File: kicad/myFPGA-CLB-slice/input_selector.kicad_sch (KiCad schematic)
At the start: 26 parts, among them U1 74AHCT595, U32 74LS153, U33 74LS153, U34 74LS153, U35 74LS153

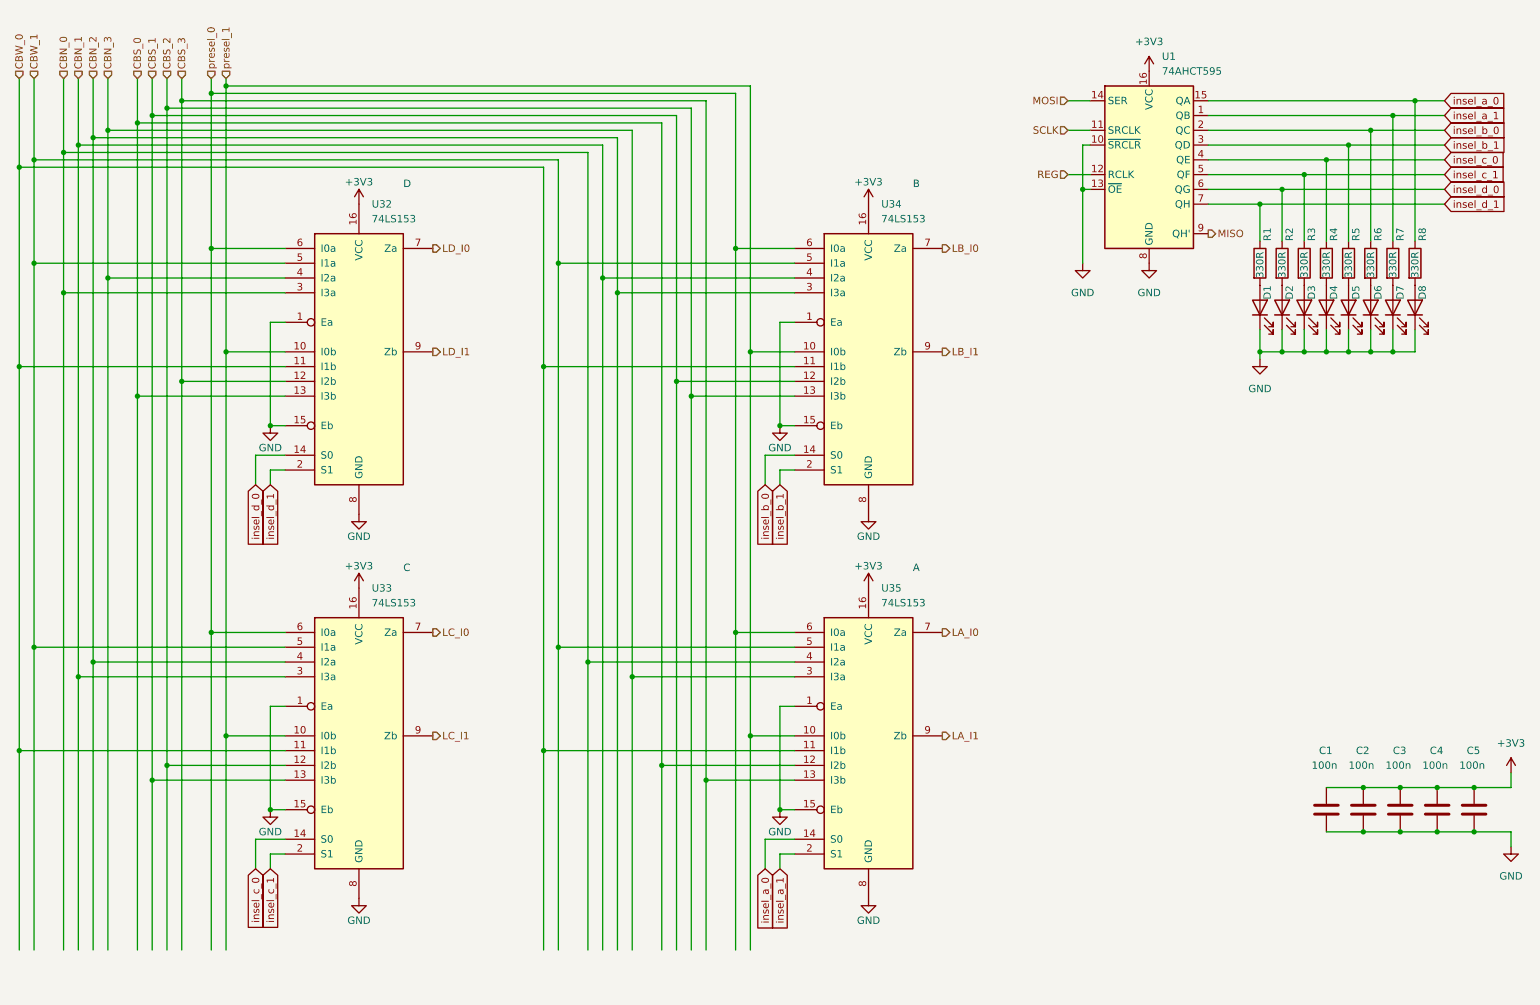
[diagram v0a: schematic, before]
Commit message: fixed kicad names, updated architecure, started CBv
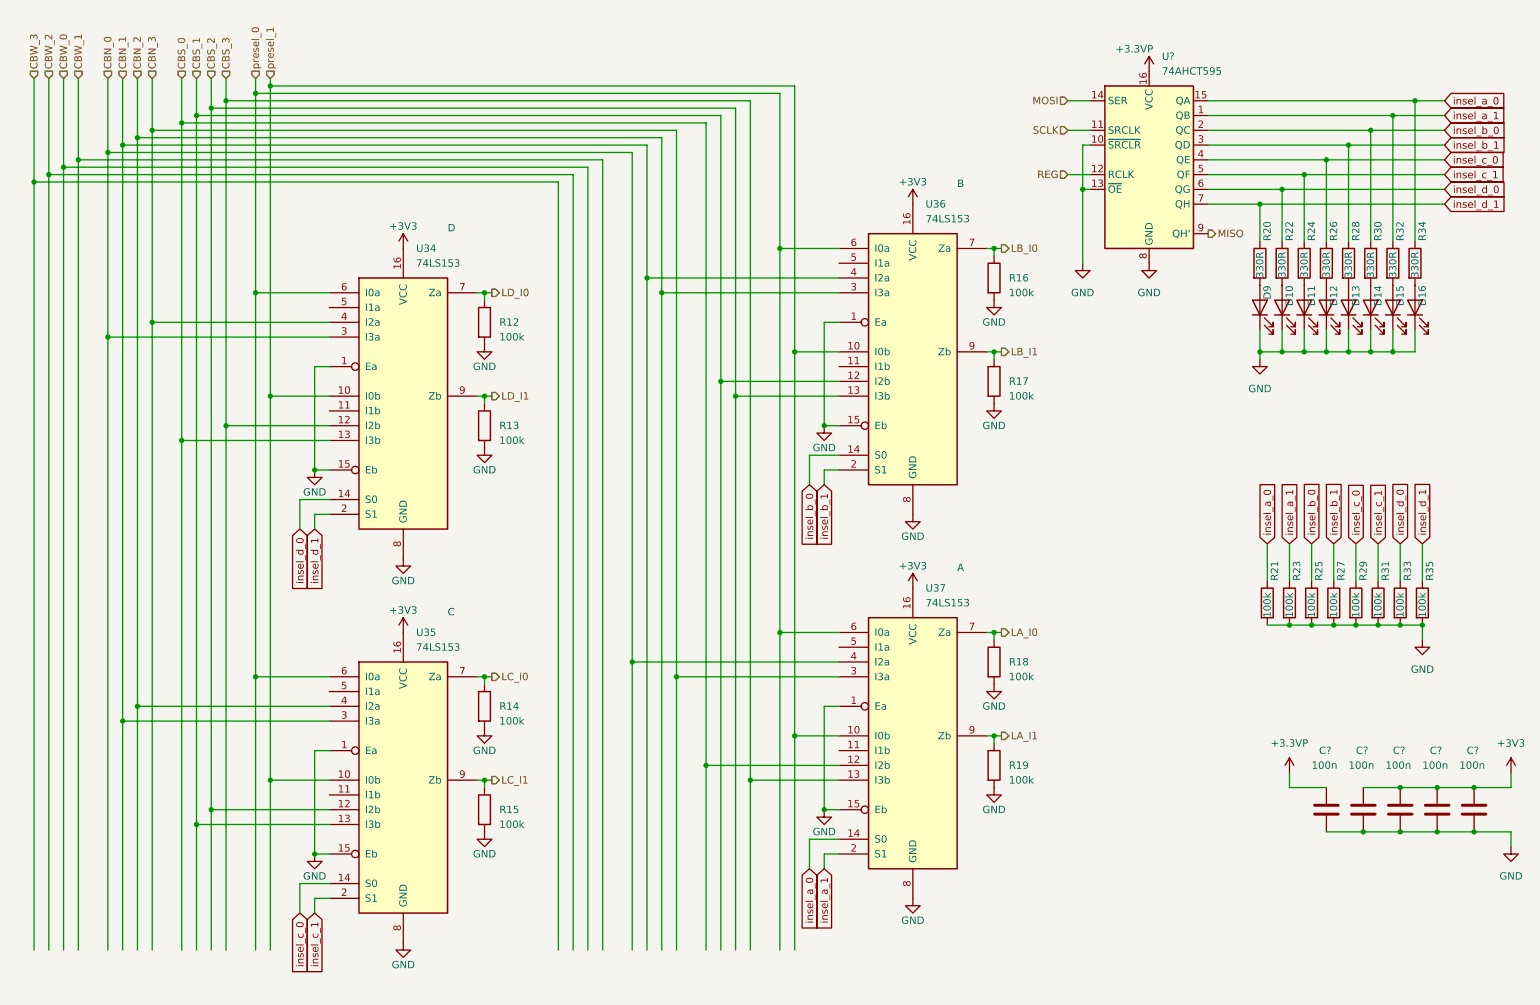
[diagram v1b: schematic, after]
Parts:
- added R12, R13, R14, R15, R16, R17, R18, R19, R21, R23, R25, R27, R29, R31, R33, R35: 100k, Resistor_SMD:R_0805_2012Metric, symbol Device:R
- C?: renamed from C4; Dielectric (none) -> X7R; JLCPCB Part # (none) -> C49678; Part Nr. (none) -> CC0805KRX7R9BB104; Voltage (none) -> 50V
- C?: renamed from C3; Dielectric (none) -> X7R; JLCPCB Part # (none) -> C49678; Part Nr. (none) -> CC0805KRX7R9BB104; Voltage (none) -> 50V
- C?: renamed from C1; Dielectric (none) -> X7R; JLCPCB Part # (none) -> C49678; Part Nr. (none) -> CC0805KRX7R9BB104; Voltage (none) -> 50V
- C?: renamed from C2; Dielectric (none) -> X7R; JLCPCB Part # (none) -> C49678; Part Nr. (none) -> CC0805KRX7R9BB104; Voltage (none) -> 50V
- C?: renamed from C5; Dielectric (none) -> X7R; JLCPCB Part # (none) -> C49678; Part Nr. (none) -> CC0805KRX7R9BB104; Voltage (none) -> 50V
- D10: renamed from D2; value LED -> LED (green); footprint (none) -> LED_SMD:LED_0805_2012Metric; JLCPCB Part # (none) -> C2297; Part Nr. (none) -> C2297
- D11: renamed from D3; value LED -> LED (green); footprint (none) -> LED_SMD:LED_0805_2012Metric; JLCPCB Part # (none) -> C2297; Part Nr. (none) -> C2297
- D12: renamed from D4; value LED -> LED (green); footprint (none) -> LED_SMD:LED_0805_2012Metric; JLCPCB Part # (none) -> C2297; Part Nr. (none) -> C2297
- D13: renamed from D5; value LED -> LED (green); footprint (none) -> LED_SMD:LED_0805_2012Metric; JLCPCB Part # (none) -> C2297; Part Nr. (none) -> C2297
- D14: renamed from D6; value LED -> LED (green); footprint (none) -> LED_SMD:LED_0805_2012Metric; JLCPCB Part # (none) -> C2297; Part Nr. (none) -> C2297
- D15: renamed from D7; value LED -> LED (green); footprint (none) -> LED_SMD:LED_0805_2012Metric; JLCPCB Part # (none) -> C2297; Part Nr. (none) -> C2297
- D16: renamed from D8; value LED -> LED (green); footprint (none) -> LED_SMD:LED_0805_2012Metric; JLCPCB Part # (none) -> C2297; Part Nr. (none) -> C2297
- D9: renamed from D1; value LED -> LED (green); footprint (none) -> LED_SMD:LED_0805_2012Metric; JLCPCB Part # (none) -> C2297; Part Nr. (none) -> C2297
- R20: renamed from R1; footprint (none) -> Resistor_SMD:R_0805_2012Metric; JLCPCB Part # (none) -> C17630; Part Nr. (none) -> 0805W8F3300T5E
- R22: renamed from R2; footprint (none) -> Resistor_SMD:R_0805_2012Metric; JLCPCB Part # (none) -> C17630; Part Nr. (none) -> 0805W8F3300T5E
- R24: renamed from R3; footprint (none) -> Resistor_SMD:R_0805_2012Metric; JLCPCB Part # (none) -> C17630; Part Nr. (none) -> 0805W8F3300T5E
- R26: renamed from R4; footprint (none) -> Resistor_SMD:R_0805_2012Metric; JLCPCB Part # (none) -> C17630; Part Nr. (none) -> 0805W8F3300T5E
- R28: renamed from R5; footprint (none) -> Resistor_SMD:R_0805_2012Metric; JLCPCB Part # (none) -> C17630; Part Nr. (none) -> 0805W8F3300T5E
- R30: renamed from R6; footprint (none) -> Resistor_SMD:R_0805_2012Metric; JLCPCB Part # (none) -> C17630; Part Nr. (none) -> 0805W8F3300T5E
- R32: renamed from R7; footprint (none) -> Resistor_SMD:R_0805_2012Metric; JLCPCB Part # (none) -> C17630; Part Nr. (none) -> 0805W8F3300T5E
- R34: renamed from R8; footprint (none) -> Resistor_SMD:R_0805_2012Metric; JLCPCB Part # (none) -> C17630; Part Nr. (none) -> 0805W8F3300T5E
- renumbered U32 to U34, U33 to U35, U34 to U36, U35 to U37, U1 to U?
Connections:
- net +3V3: no longer C?.1, U?.16 (VCC)
- net CBW_0: no longer U34.11 (I1b), U35.11 (I1b), U36.11 (I1b), U37.11 (I1b)
- net CBW_1: no longer U34.5 (I1a), U35.5 (I1a), U36.5 (I1a), U37.5 (I1a)
- net GND: now also R12.2, R13.2, R14.2, R15.2, R16.2, R17.2, R18.2, R19.2, R21.2, R23.2, R25.2, R27.2, R29.2, R31.2, R33.2, R35.2
- net LA_I0: now also R18.1
- net LA_I1: now also R19.1
- net LB_I0: now also R16.1
- net LB_I1: now also R17.1
- net LC_I0: now also R14.1
- net LC_I1: now also R15.1
- net LD_I0: now also R12.1
- net LD_I1: now also R13.1
- net insel_a_0: now also R21.1
- net insel_a_1: now also R23.1
- net insel_b_0: now also R25.1
- net insel_b_1: now also R27.1
- net insel_c_0: now also R29.1
- net insel_c_1: now also R31.1
- net insel_d_0: now also R33.1
- net insel_d_1: now also R35.1
- new net +3.3VP: C?.1, U?.16 (VCC)
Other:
- moved on the sheet: U34, U35, U36, U37
